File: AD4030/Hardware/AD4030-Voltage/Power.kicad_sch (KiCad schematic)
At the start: 51 parts, among them J501 1715721, Q501 SI5618A, Q502 MMBT3904, U501 TPS65133DPDR, U502 TSR_1-2433, U503 TEC3-2419WI, U504 LT1763CDE-ADJ, U505 LT1763CDE-1.8, U506 LT1763IDE-3.3, U507 TSR_1-2450

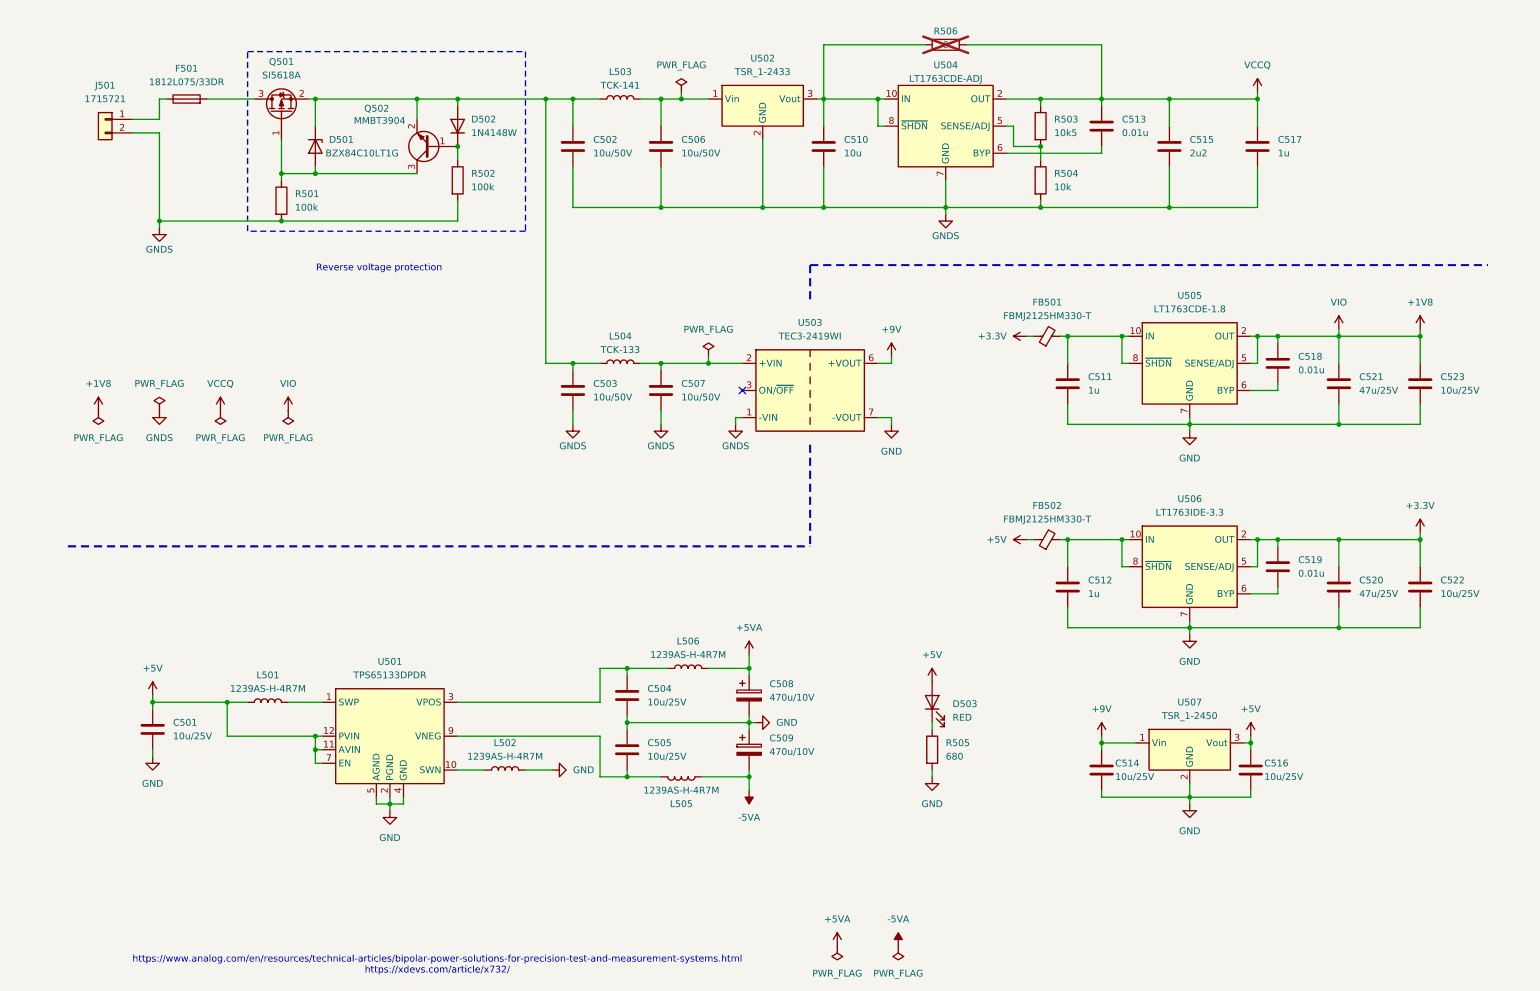
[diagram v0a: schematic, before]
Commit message: PCB layout
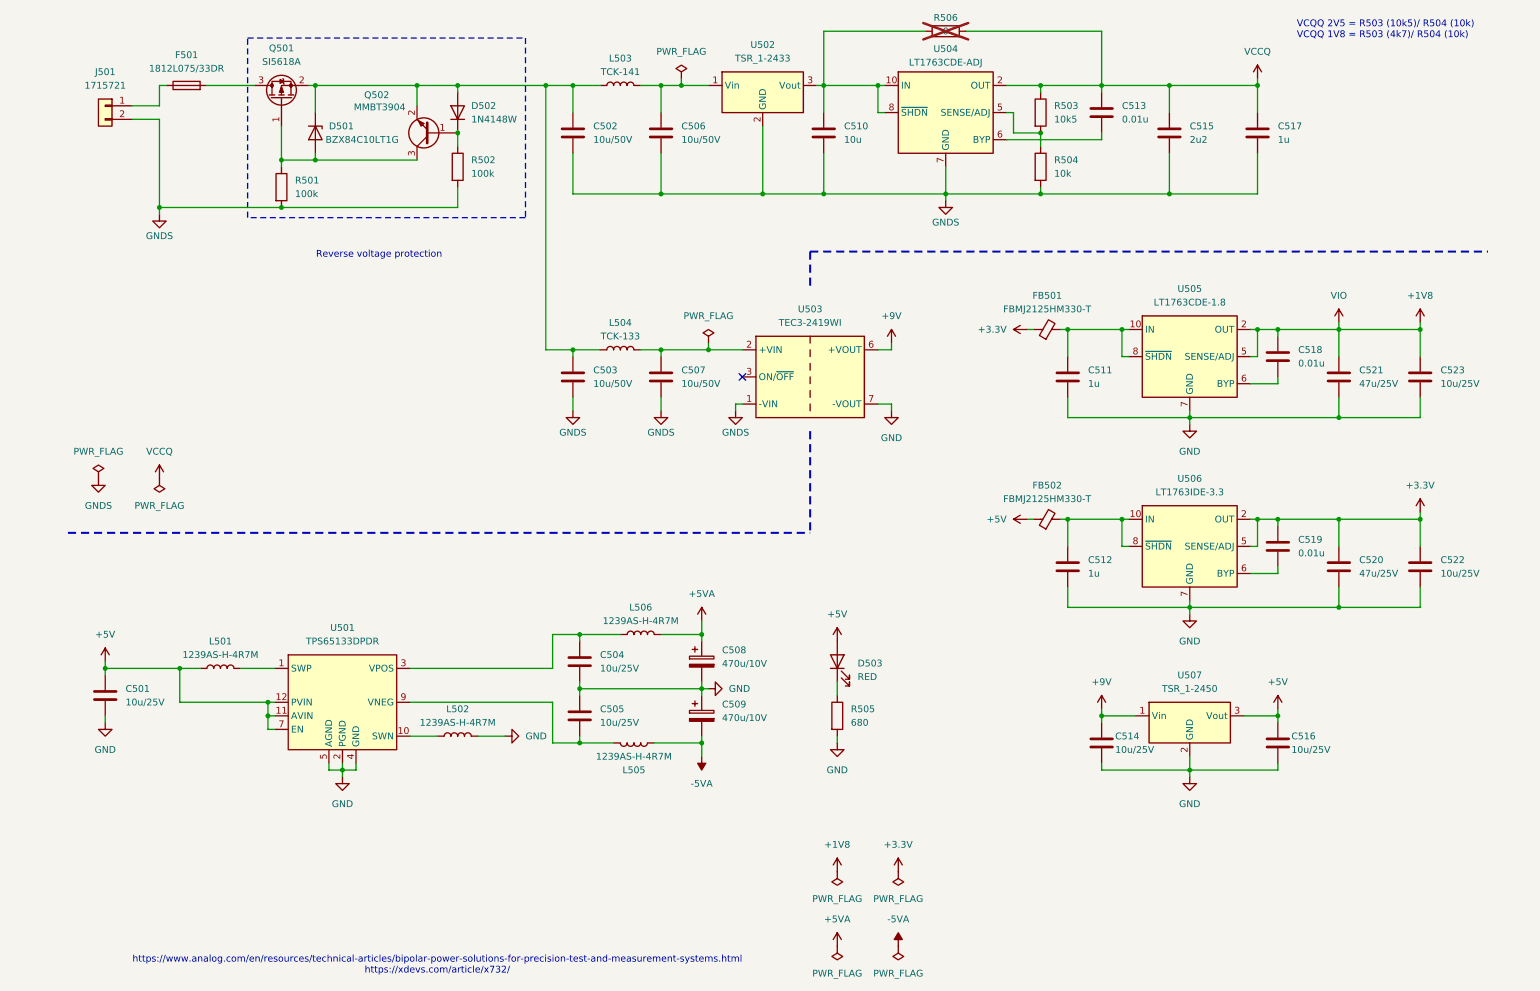
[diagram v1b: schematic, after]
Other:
- note added: "VCQQ 2V5 = R503 (10k5)/ R504 (10k) VCQQ 1V8 = R503 (4k7)/ R504 (10k)"
- moved on the sheet: C501, C502, C503, C504, C505, C506, C507, C508, C509, C510, C511, C512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
